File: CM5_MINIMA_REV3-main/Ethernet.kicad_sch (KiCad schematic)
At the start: 7 parts, among them J1 GLPLX-SMT-188S7, U401 TPD4EUSB30, U402 TPD4EUSB30

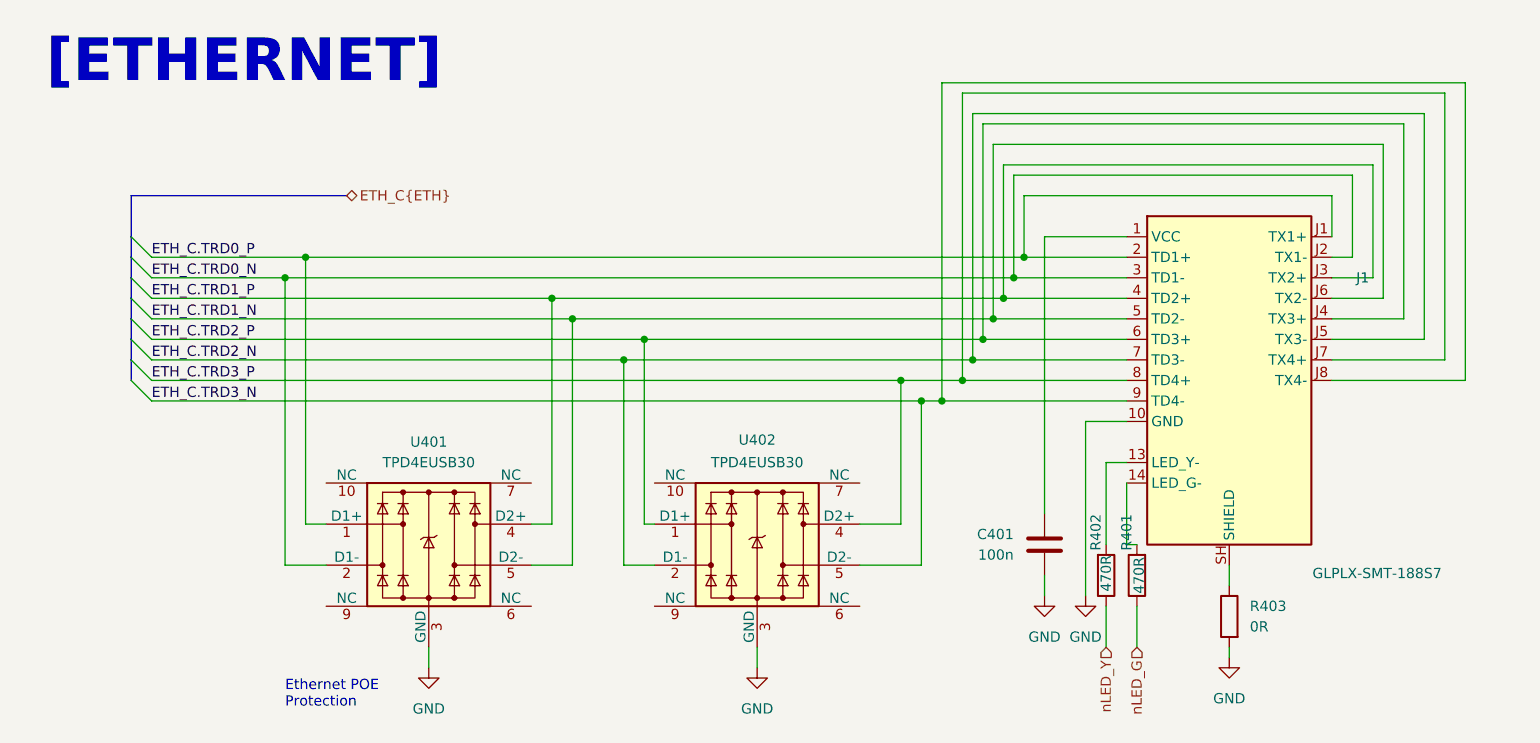
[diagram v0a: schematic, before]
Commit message: Revert CM5_MINIMA_REV3-main to pre-warning-fix state (feae2c2) - fix component mismatches
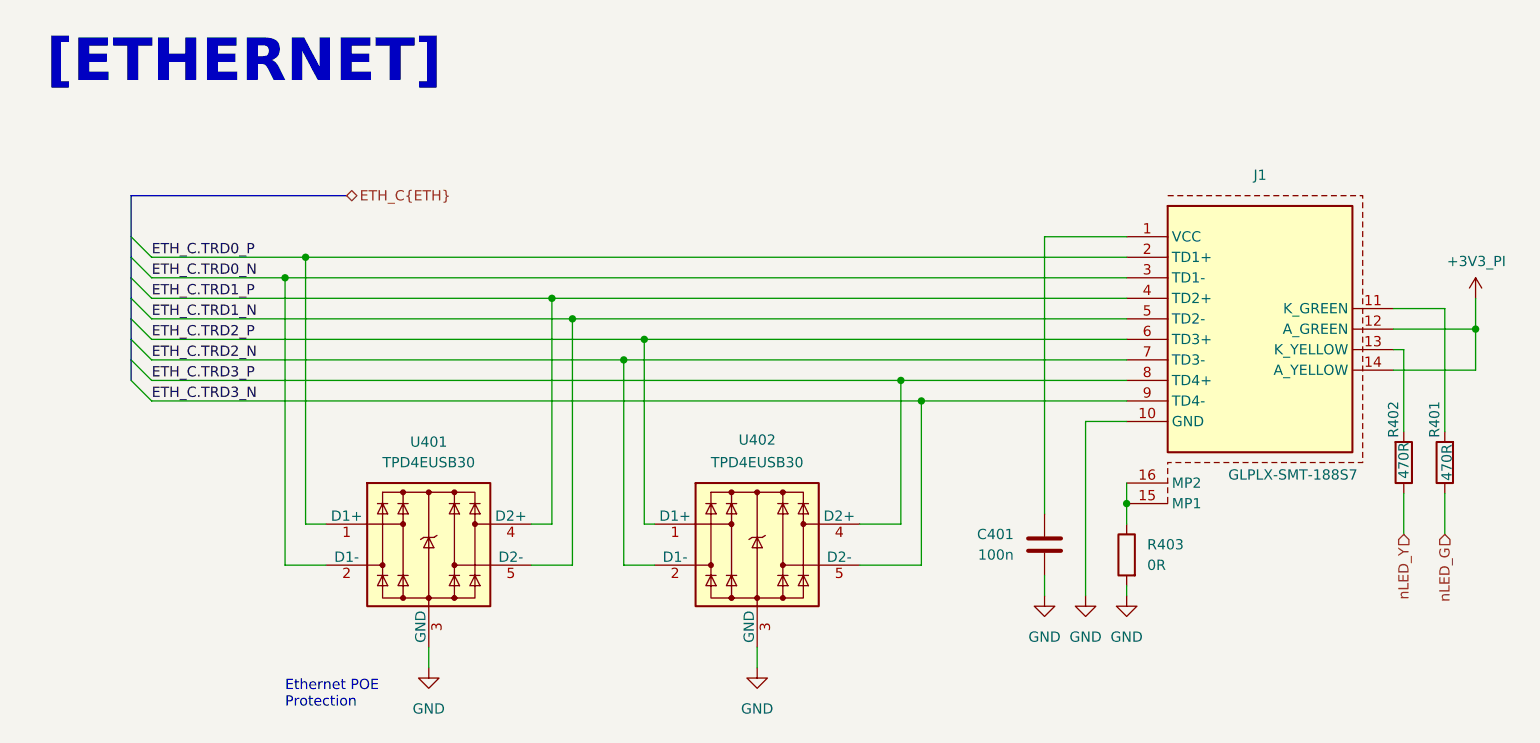
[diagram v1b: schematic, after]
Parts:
- J1: footprint CM5_MINIMA_local:GLPLXSMT188S7QQYG -> Samacsys:GLPLXSMT188S7QQYG; MPN GLPLX-SMT-188S7-QQ-Y/G -> (none); Manufacturer Kycon -> (none)
- U401, U402: symbol Power_Protection:TPD4EUSB30 -> CM4IO:TPD4EUSB30
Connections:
- net ETH_C.TRD0_N: now also U401.9; no longer J1.J2 (TX1-)
- net ETH_C.TRD0_P: now also U401.10; no longer J1.J1 (TX1+)
- net ETH_C.TRD1_N: now also U401.6; no longer J1.J6 (TX2-)
- net ETH_C.TRD1_P: now also U401.7; no longer J1.J3 (TX2+)
- net ETH_C.TRD2_N: now also U402.9; no longer J1.J5 (TX3-)
- net ETH_C.TRD2_P: now also U402.10; no longer J1.J4 (TX3+)
- net ETH_C.TRD3_N: now also U402.6; no longer J1.J8 (TX4-)
- net ETH_C.TRD3_P: now also U402.7; no longer J1.J7 (TX4+)
- net at R401.2: now also J1.11 (K_GREEN); no longer J1.14 (LED_G-)
- net at R403.1: now also J1.15 (MP1), J1.16 (MP2); no longer J1.SH (SHIELD)
- new net +3V3_PI: J1.12 (A_GREEN), J1.14 (A_YELLOW)
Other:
- moved on the sheet: R401, R402, R403
